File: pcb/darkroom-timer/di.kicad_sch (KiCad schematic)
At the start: 8 parts, among them SW2 SW_Rotary_1x3_MP, SW3 SW_Rotary_1x3_MP

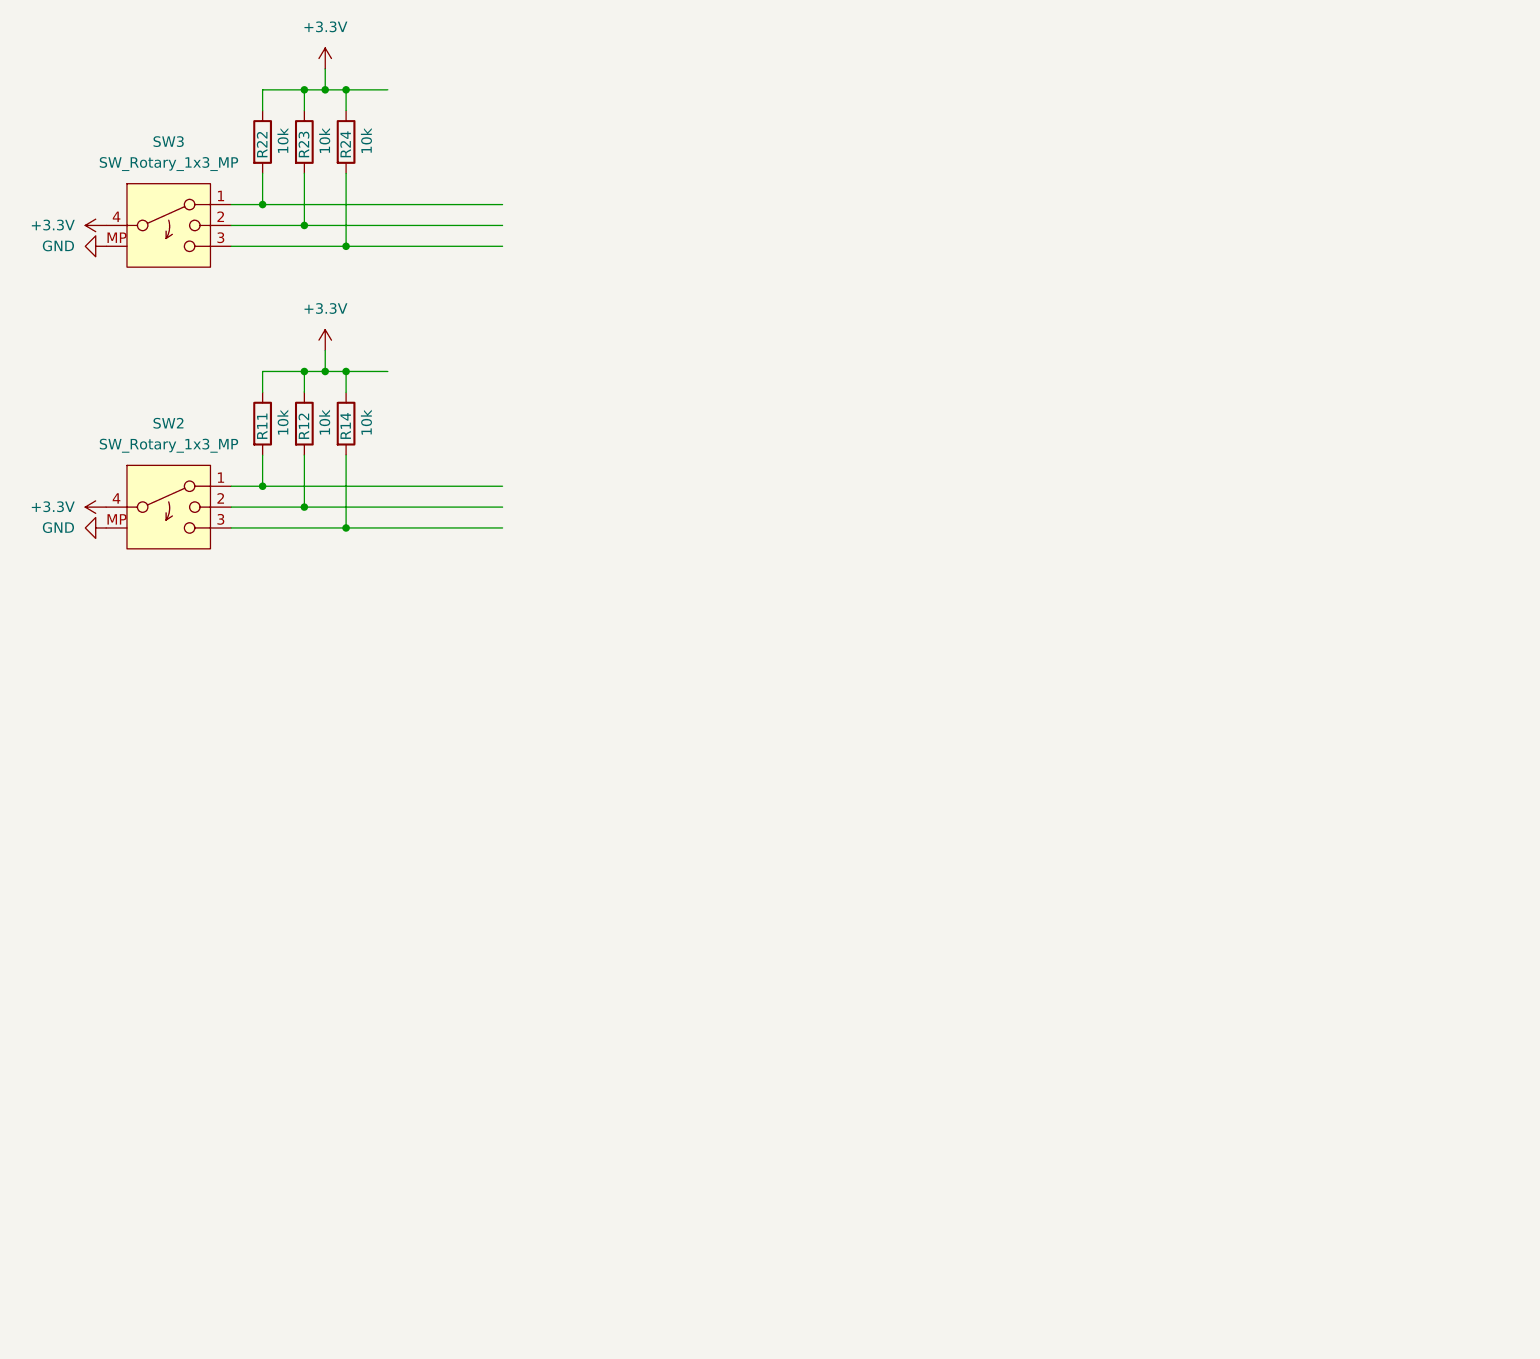
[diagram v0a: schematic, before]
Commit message: PCB Ready
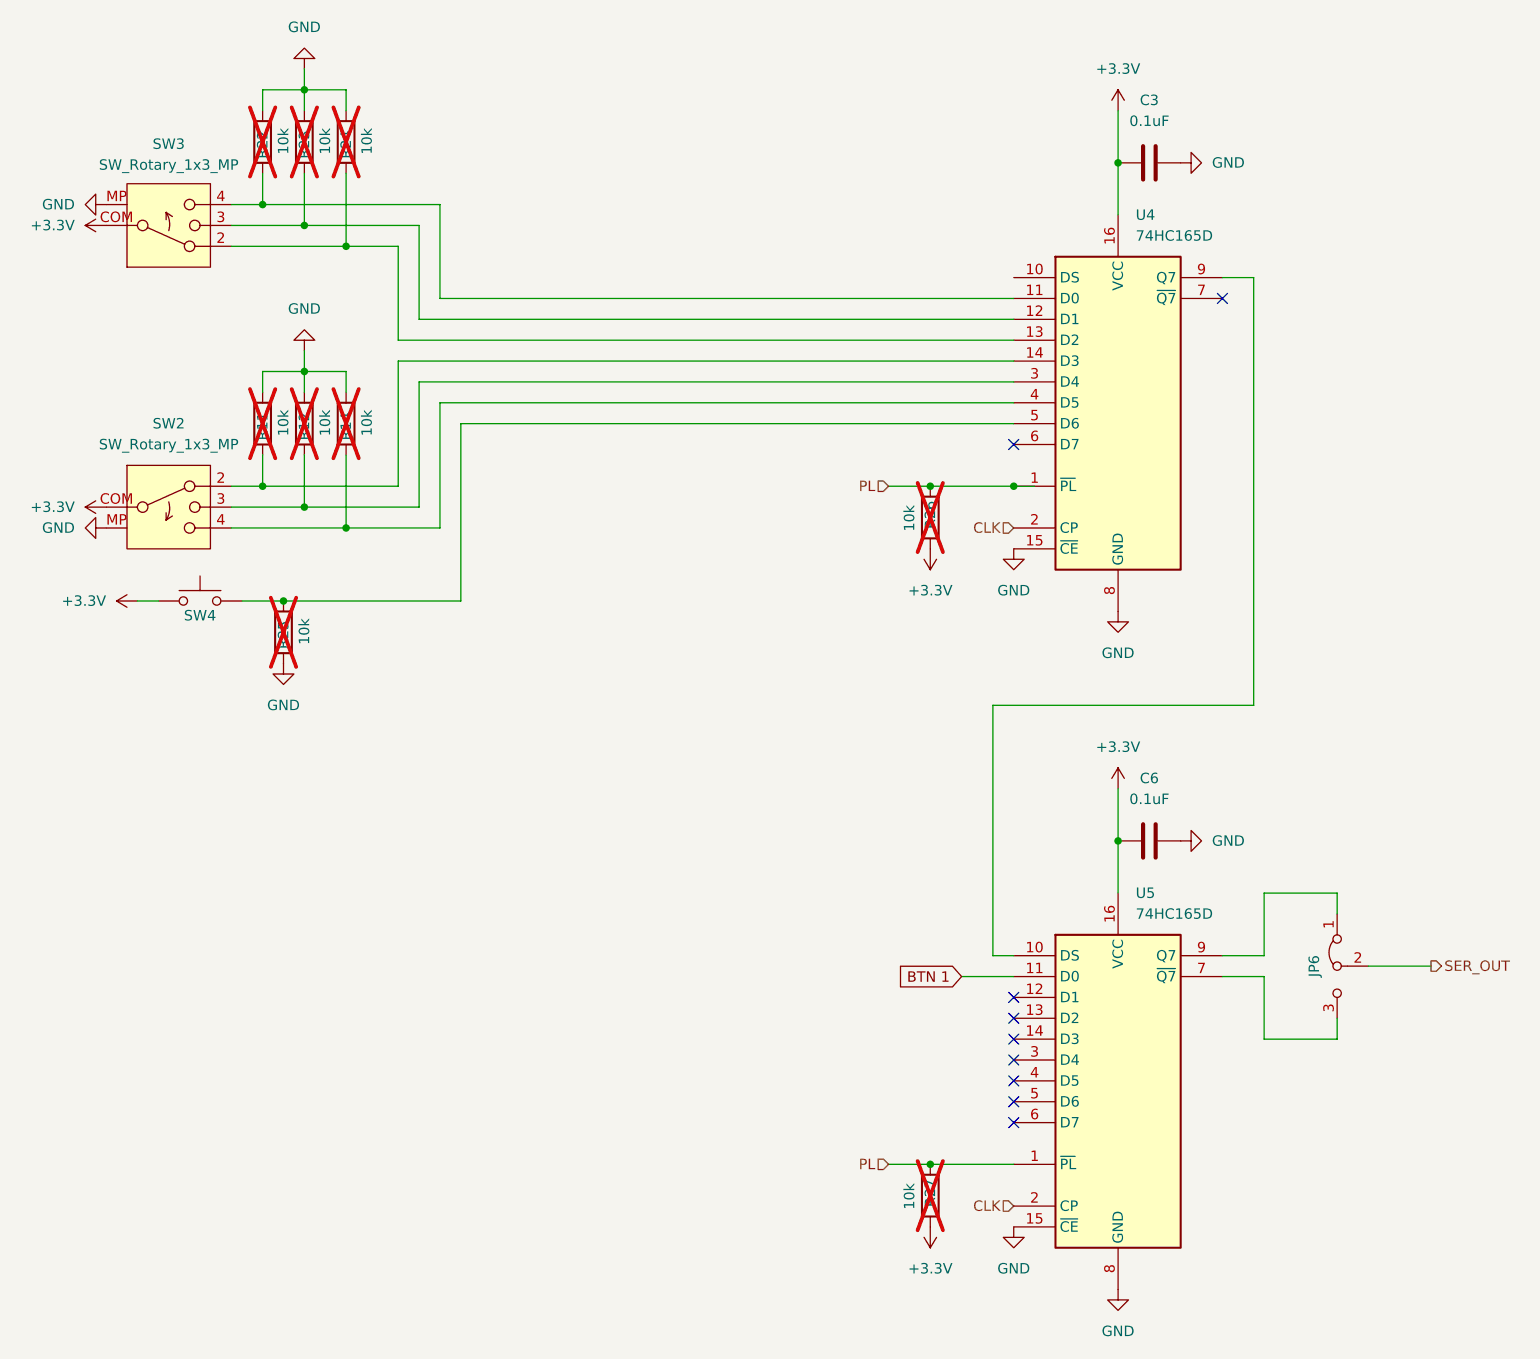
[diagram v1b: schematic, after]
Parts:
- added C3, C6: 0.1uF, Capacitor_SMD:C_0805_2012Metric, symbol Device:C
- added JP6: ~, Jumper:SolderJumper-3_P1.3mm_Bridged12_Pad1.0x1.5mm, symbol Jumper:Jumper_3_Bridged12
- added R25, R26, R27: 10k, Resistor_SMD:R_0805_2012Metric, symbol Device:R
- added SW4: Start Switch, Connector_Wire:SolderWire-0.25sqmm_1x02_P4.5mm_D0.65mm_OD2mm, symbol Switch:SW_Push
- added U4, U5: 74HC165D, Package_SO:SO-16_3.9x9.9mm_P1.27mm, symbol 74xx:74HC165
- R11, R12, R14, R22, R23, R24: footprint Resistor_SMD:R_0201_0603Metric -> Resistor_SMD:R_0805_2012Metric; Placement Optional -> (none); now not fitted
- SW2, SW3: footprint (none) -> Frank:SR17A-007; InvenTree Part # (none) -> 543; Placement Required -> (none)
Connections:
- net +3.3V: now also SW2.COM, SW3.COM, C3.1, C6.1, R26.1, R27.1, SW4.1, U4.16 (VCC), U5.16 (VCC); no longer R11.1, R12.1, R14.1, R22.1, R23.1, R24.1, SW2.4, SW3.4
- net GND: now also R11.1, R12.1, R14.1, R22.1, R23.1, R24.1, C3.2, C6.2, R25.2, U4.15 (~{CE}), U4.8 (GND), U5.15 (~{CE}), U5.8 (GND)
- net at R24.2: now also SW3.2, U4.13 (D2); no longer SW3.3
- net at R14.2: now also SW2.4, U4.4 (D5); no longer SW2.3
- net at R22.2: now also SW3.4, U4.11 (D0); no longer SW3.1
- net at R23.2: now also SW3.3, U4.12 (D1); no longer SW3.2
- net at R11.2: now also SW2.2, U4.14 (D3); no longer SW2.1
- net at R12.2: now also SW2.3, U4.3 (D4); no longer SW2.2
- new net: JP6.1 (A), U5.9 (Q7)
- new net: JP6.3 (B), U5.7 (~{Q7})
- new net: R25.1, SW4.2, U4.5 (D6)
- new net: U4.9 (Q7), U5.10 (DS)
- new net BTN 1: U5.11 (D0)
- new net CLK: U4.2 (CP), U5.2 (CP)
- new net PL: R26.2, R27.2, U4.1 (~{PL}), U5.1 (~{PL})
- new net SER_OUT: JP6.2 (C)
- no-connect marks 0 -> 9

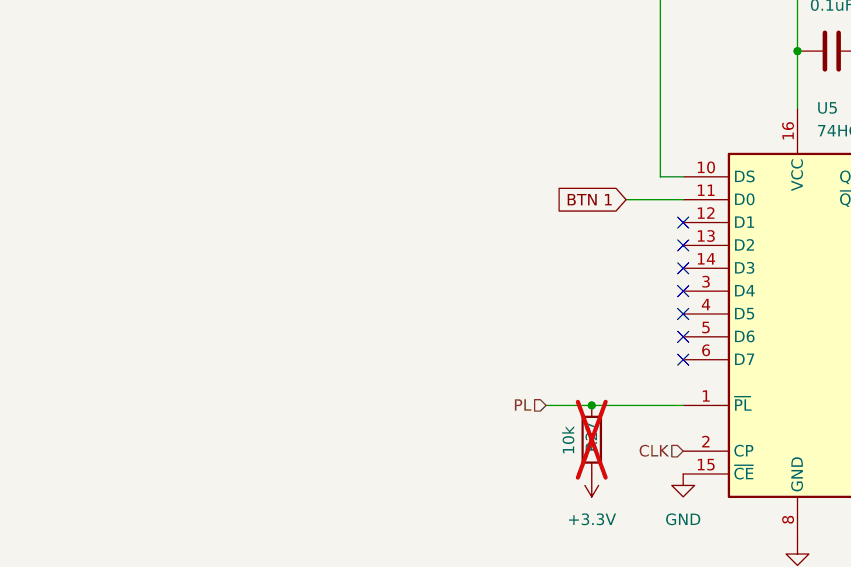
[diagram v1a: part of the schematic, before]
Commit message: Final PCB R0 design
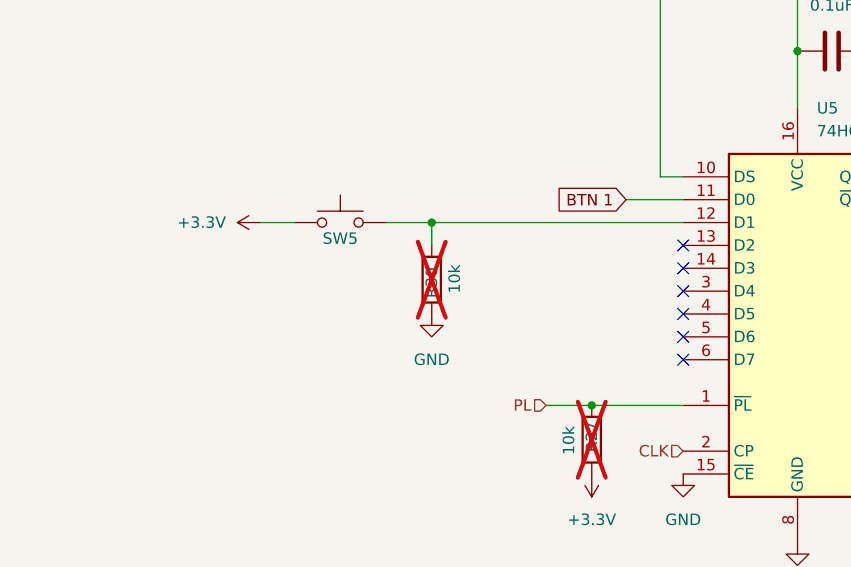
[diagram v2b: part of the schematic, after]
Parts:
- added R30: 10k, Resistor_SMD:R_0805_2012Metric, symbol Device:R
- added SW5: Start Switch, Button_Switch_THT:SW_PUSH_6mm_H13mm, symbol Switch:SW_Push
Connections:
- net +3.3V: now also SW5.1
- net GND: now also R30.2
- net at U5.12 (D1): now also R30.1, SW5.2
- no-connect marks 9 -> 8
